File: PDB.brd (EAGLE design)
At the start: 159.7 x 150.8 mm, 76 parts, among them IC1 LM555N

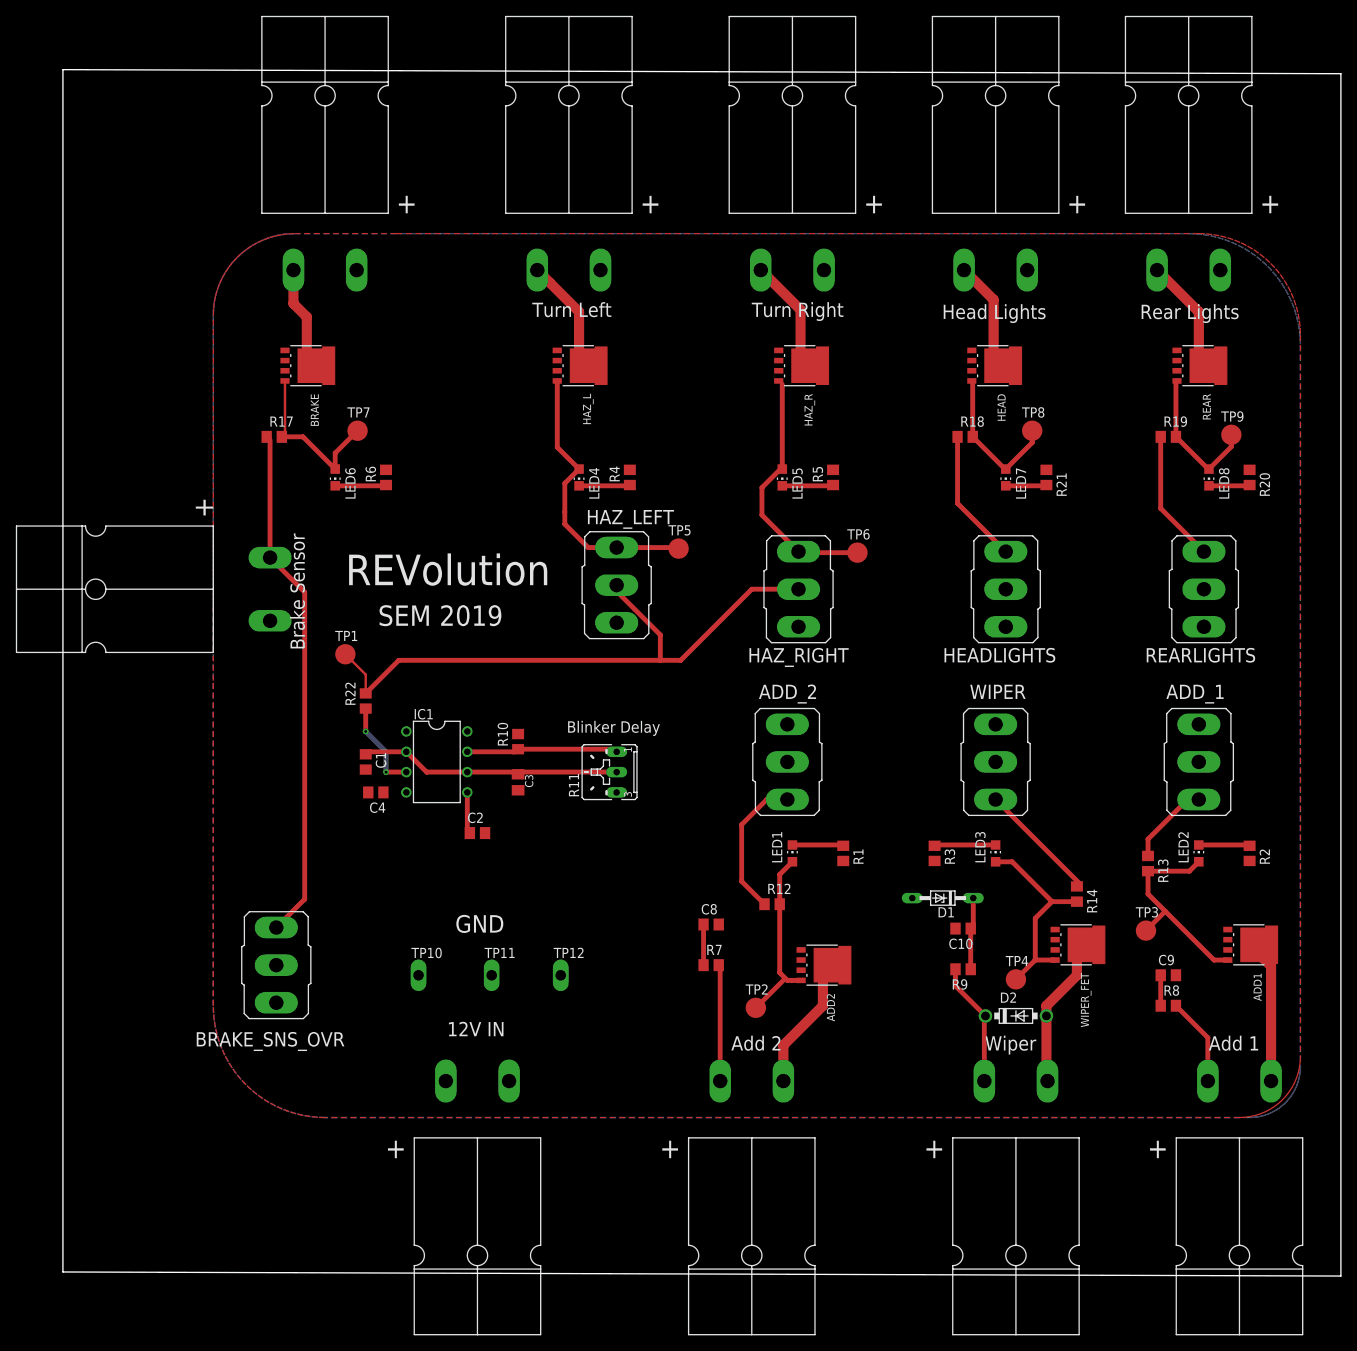
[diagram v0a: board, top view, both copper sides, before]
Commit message: added stuff to pdb
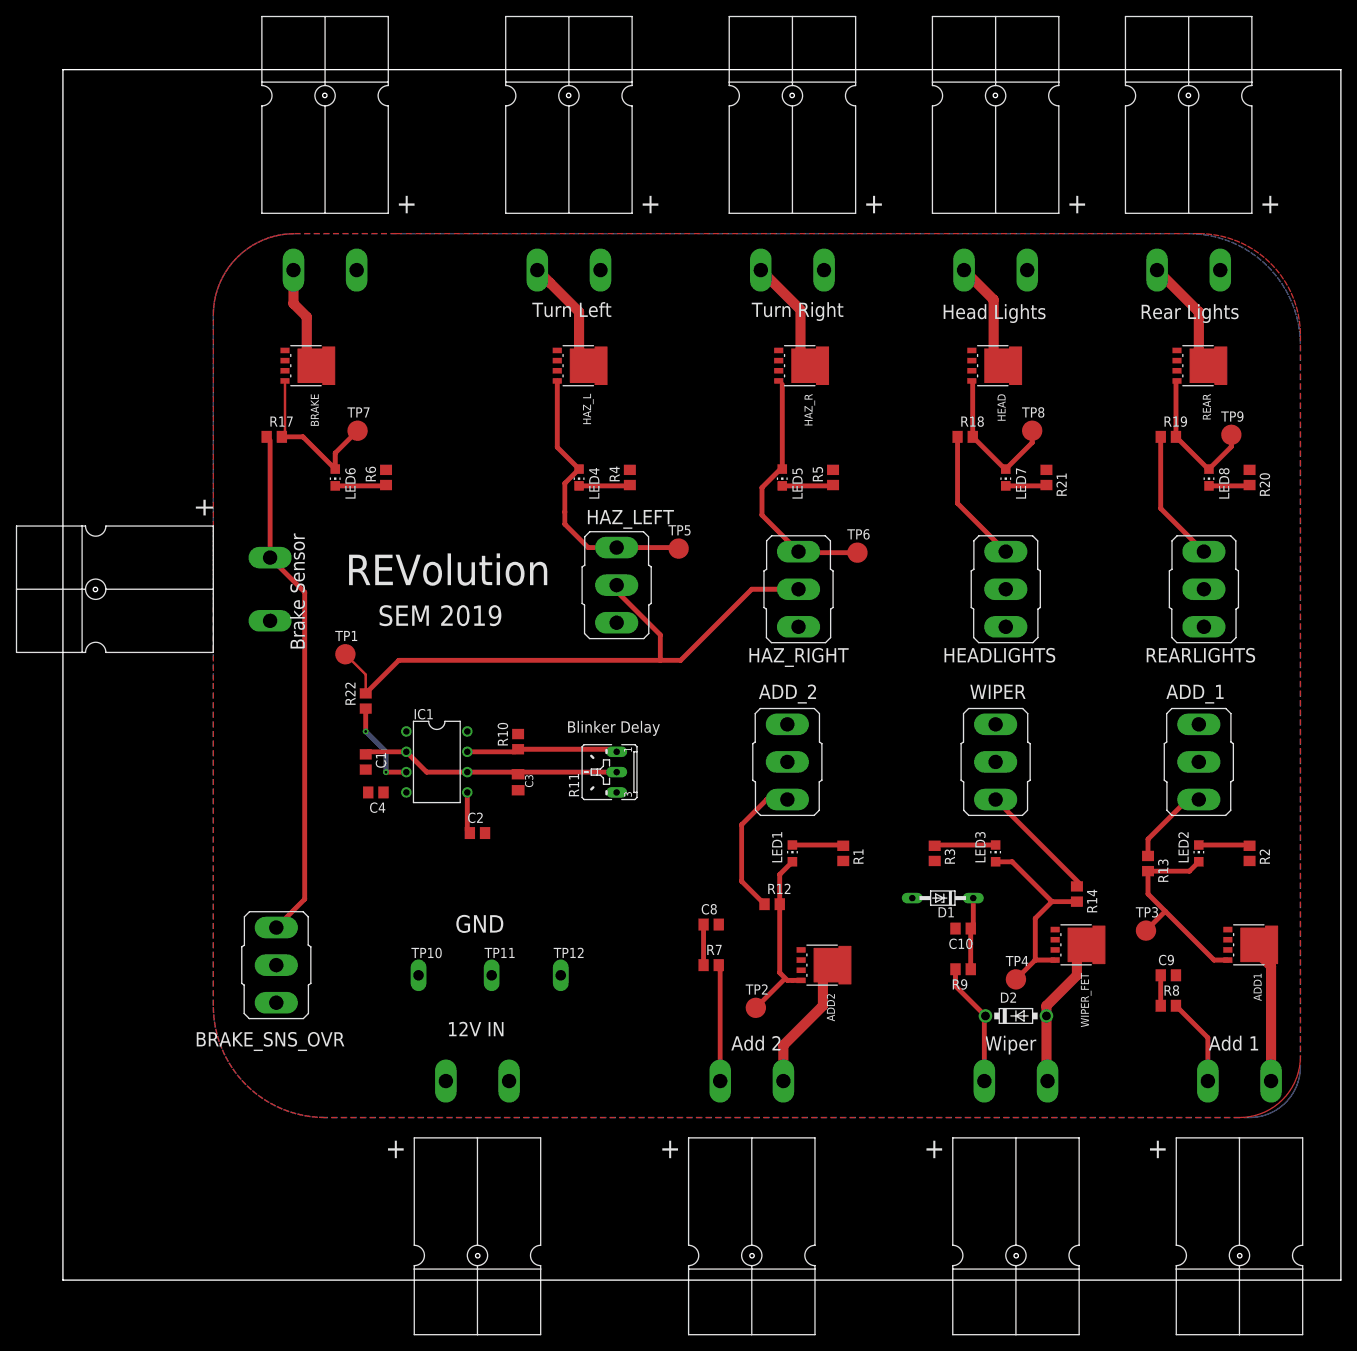
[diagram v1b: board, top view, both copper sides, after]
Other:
- board size 159.7 x 150.8 mm -> 159.7 x 151.3 mm
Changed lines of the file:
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@@
 <board>
 <plain>
-<wire x1="-2.286" y1="-21.844" x2="157.46" y2="-22.352" width="0" layer="20"/>
-<wire x1="157.46" y1="-22.352" x2="157.46" y2="127.94" width="0" layer="20"/>
-<wire x1="157.46" y1="127.94" x2="-2.286" y2="128.448" width="0" layer="20"/>
-<wire x1="-2.286" y1="128.448" x2="-2.286" y2="-21.844" width="0" layer="20"/>
+<wire x1="-2.286" y1="-22.86" x2="157.46" y2="-22.86" width="0" layer="20"/>
+<wire x1="157.46" y1="-22.86" x2="157.46" y2="128.448" width="0" layer="20"/>
+<wire x1="157.46" y1="128.448" x2="-2.286" y2="128.448" width="0" layer="20"/>
+<wire x1="-2.286" y1="128.448" x2="-2.286" y2="-22.86" width="0" layer="20"/>
 <text x="46.736" y="20.574" size="2.1844" layer="25">GND</text>
 <text x="45.72" y="7.62" size="1.778" layer="25">12V IN </text>
